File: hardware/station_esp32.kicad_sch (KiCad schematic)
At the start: 8 parts, among them J1 Conn_01x04, U1 DHT11, U2 ESP32-WROOM-32

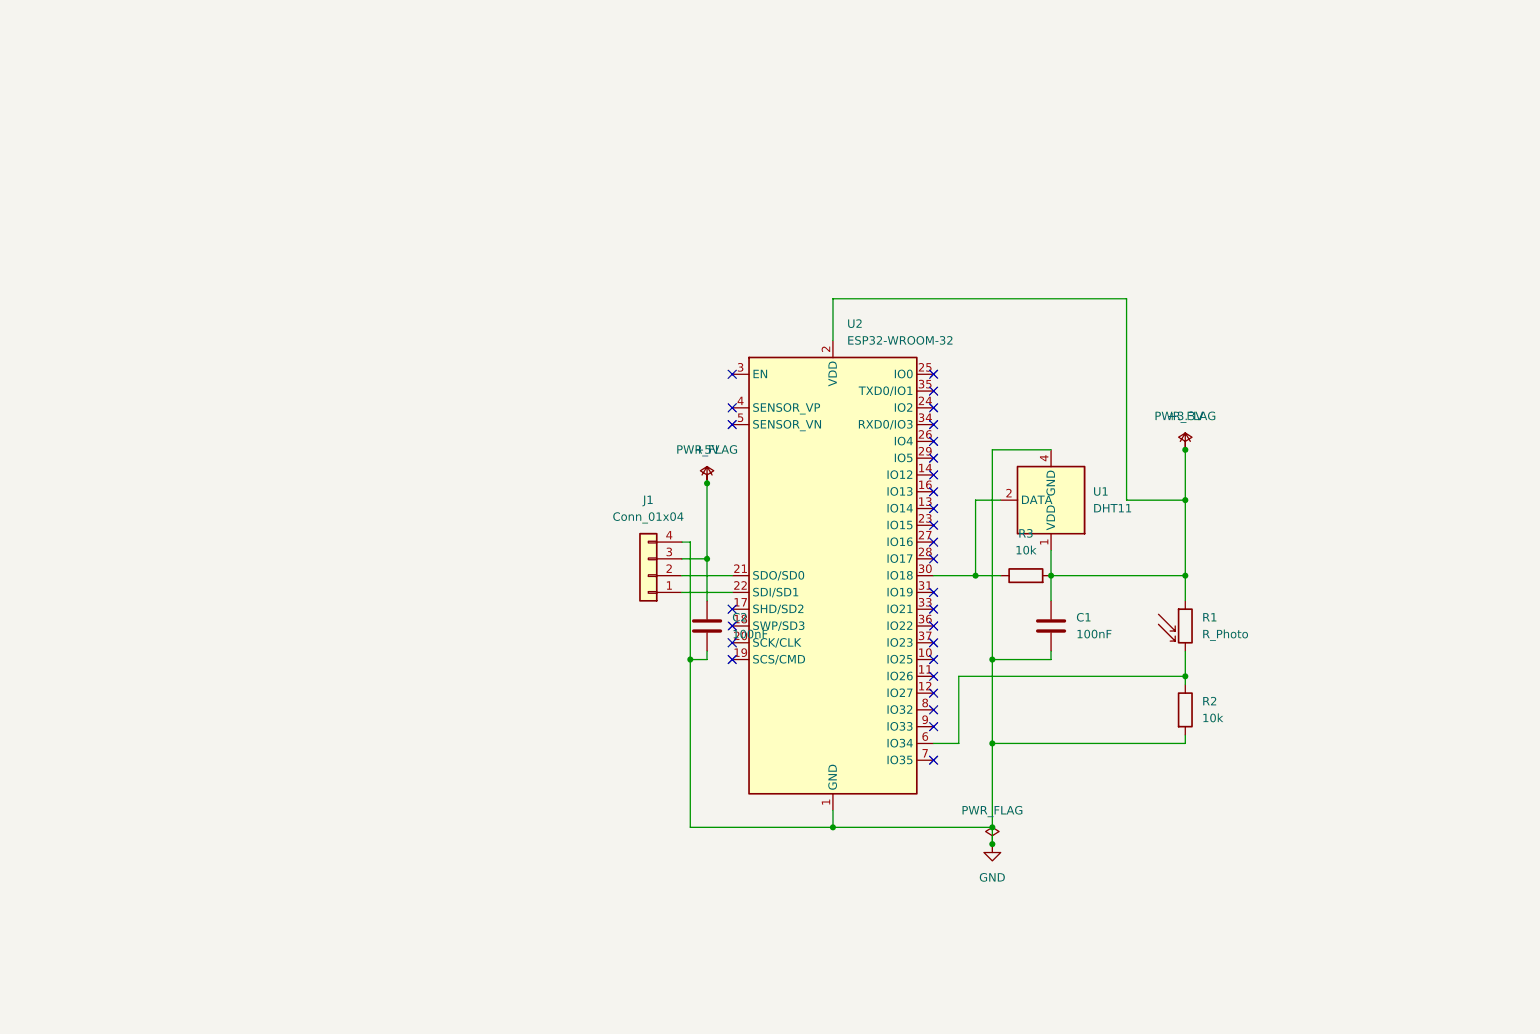
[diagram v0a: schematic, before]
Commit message: Add files via upload
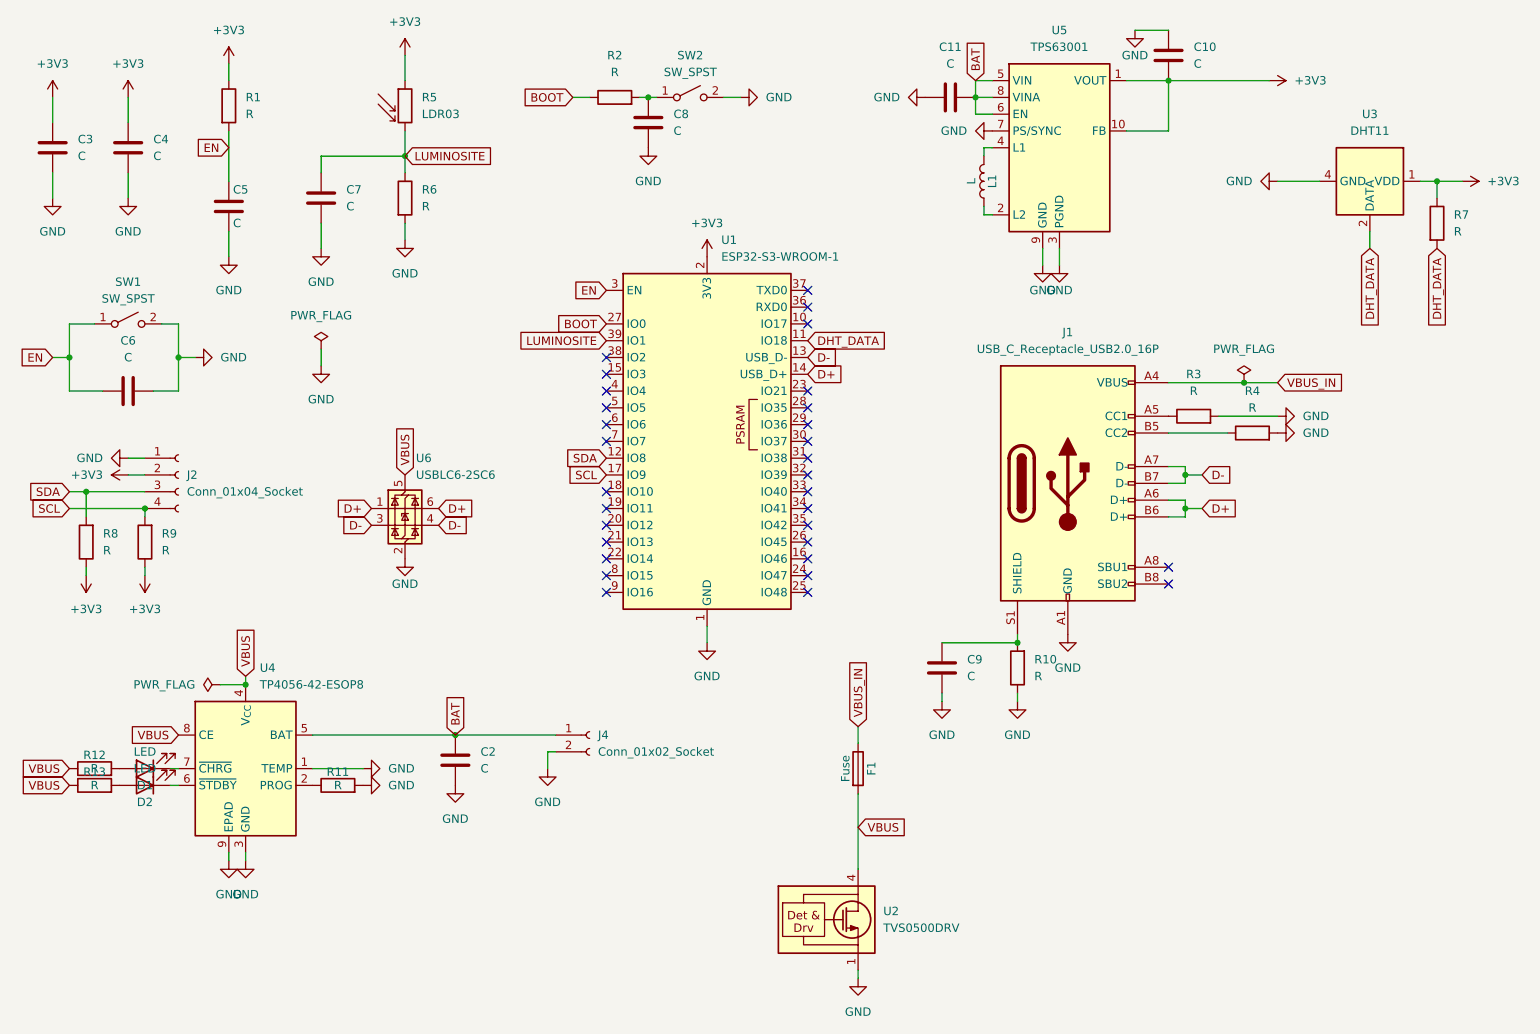
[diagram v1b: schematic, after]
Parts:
- removed C1: 100nF, Capacitor_THT:C_Disc_D5.0mm_W2.5mm_P5.00mm, symbol Device:C
- removed J1: Conn_01x04, Connector_PinHeader_2.54mm:PinHeader_1x04_P2.54mm_Vertical, symbol Connector_Generic:Conn_01x04
- removed R1: R_Photo, OptoDevice:R_LDR_5.0x4.1mm_P3mm_Vertical, symbol Device:R_Photo
- removed U1: DHT11, Sensor:Aosong_DHT11_5.5x12.0_P2.54mm, symbol Sensor:DHT11
- removed U2: ESP32-WROOM-32, RF_Module:ESP32-WROOM-32, symbol RF_Module:ESP32-WROOM-32
- added C10, C11, C3, C4, C5, C6, C7, C8, C9: C, Capacitor_SMD:C_0805_2012Metric, symbol Device:C
- added D1, D2: LED, LED_SMD:LED_0805_2012Metric, symbol Device:LED
- added F1: Fuse, Fuse:Fuse_0805_2012Metric, symbol Device:Fuse
- added J1: USB_C_Receptacle_USB2.0_16P, Connector_USB:USB_C_Receptacle_GCT_USB4105-xx-A_16P_TopMnt_Horizontal, symbol Connector:USB_C_Receptacle_USB2.0_16P
- added J2: Conn_01x04_Socket, Connector_JST:JST_PH_B4B-PH-K_1x04_P2.00mm_Vertical, symbol Connector:Conn_01x04_Socket
- added J4: Conn_01x02_Socket, Connector_JST:JST_PH_B2B-PH-K_1x02_P2.00mm_Vertical, symbol Connector:Conn_01x02_Socket
- added L1: L, Inductor_SMD:L_0805_2012Metric, symbol Device:L
- added R1, R10, R11, R12, R13, R4, R6, R7, R8, R9: R, Resistor_SMD:R_0805_2012Metric, symbol Device:R
- added R5: LDR03, OptoDevice:R_LDR_10x8.5mm_P7.6mm_Vertical, symbol Sensor_Optical:LDR03
- added SW1, SW2: SW_SPST, Button_Switch_SMD:SW_SPST_B3U-1000P, symbol Switch:SW_SPST
- added U1: ESP32-S3-WROOM-1, RF_Module:ESP32-S3-WROOM-1, symbol RF_Module:ESP32-S3-WROOM-1
- added U2: TVS0500DRV, Package_SON:WSON-6-1EP_2x2mm_P0.65mm_EP1x1.6mm, symbol Power_Protection:TVS0500DRV
- added U3: DHT11, Sensor:Aosong_DHT11_5.5x12.0_P2.54mm, symbol Sensor:DHT11
- added U4: TP4056-42-ESOP8, Package_SO:SOIC-8-1EP_3.9x4.9mm_P1.27mm_EP2.41x3.3mm_ThermalVias, symbol Battery_Management:TP4056-42-ESOP8
- added U5: TPS63001, Package_SON:Texas_DRC0010J_ThermalVias, symbol Regulator_Switching:TPS63001
- added U6: USBLC6-2SC6, Package_TO_SOT_SMD:SOT-23-6, symbol Power_Protection:USBLC6-2SC6
- C2: value 100nF -> C; footprint Capacitor_THT:C_Disc_D5.0mm_W2.5mm_P5.00mm -> Capacitor_SMD:C_0805_2012Metric
- R2, R3: value 10k -> R; footprint Resistor_THT:R_Axial_DIN0207_L6.3mm_D2.5mm_P10.16mm_Horizontal -> Resistor_SMD:R_0805_2012Metric
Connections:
- net +3.3V is gone; now on net GND: R3.2
- net GND: now also C10.1, C11.1, C3.2, C4.2, C5.2, C6.2, C7.2, C8.2, C9.2, J1.A1 (GND), J1.A12 (GND), J1.B1 (GND), J1.B12 (GND), J2.1 (Pin_1), J4.2 (Pin_2), R10.1, R11.2, R4.2, R6.2, SW1.2 (B), SW2.2 (B), U1.1 (GND), U1.40 (GND), U1.41 (GND), U2.1 (GND), U2.2 (GND), U2.3 (GND), U2.7 (GND), U3.4 (GND), U4.1 (TEMP), U4.3 (GND), U4.9 (EPAD), U5.11 (PGND), U5.3 (PGND), U5.7 (PS/SYNC), U5.9 (GND), U6.2 (GND); no longer R2.2
- net BOOT: now reaches R2.1
- net BOOT: now also U1.27 (IO0)
- net at R3.1: now also J1.A5 (CC1)
- net +5V renamed BAT
- net BAT: now also C11.2, J4.1 (Pin_1), U4.5 (BAT), U5.5 (VIN), U5.6 (EN), U5.8 (VINA)
- new net: C8.1, R2.2, SW2.1 (A)
- new net: D2.2 (A), R13.2
- new net: L1.1, U5.2 (L2)
- new net: L1.2, U5.4 (L1)
- new net: R11.1, U4.2 (PROG)
- new net: D1.2 (A), R12.2
- new net: D1.1 (K), U4.7 (~{CHRG})
- new net: J1.B5 (CC2), R4.1
- new net: C9.1, J1.S1 (SHIELD), R10.2
- new net: D2.1 (K), U4.6 (~{STDBY})
- new net +3V3: C10.2, C3.1, C4.1, J2.2 (Pin_2), R1.1, R5.1, R7.1, R8.1, R9.1, U1.2 (3V3), U3.1 (VDD), U5.1 (VOUT), U5.10 (FB)
- new net D+: J1.A6 (D+), J1.B6 (D+), U1.14 (USB_D+), U6.1 (I/O1), U6.6 (I/O1)
- new net D-: J1.A7 (D-), J1.B7 (D-), U1.13 (USB_D-), U6.3 (I/O2), U6.4 (I/O2)
- new net DHT_DATA: R7.2, U1.11 (IO18), U3.2 (DATA)
- new net EN: C5.1, C6.1, R1.2, SW1.1 (A), U1.3 (EN)
- new net LUMINOSITE: C7.1, R5.2, R6.1, U1.39 (IO1)
- new net SCL: J2.4 (Pin_4), R9.2, U1.17 (IO9)
- new net SDA: J2.3 (Pin_3), R8.2, U1.12 (IO8)
- new net VBUS: F1.2, R12.1, R13.1, U2.4 (IN), U2.5 (IN), U2.6 (IN), U4.4 (V_{CC}), U4.8 (CE), U6.5 (VBUS)
- new net VBUS_IN: F1.1, J1.A4 (VBUS), J1.A9 (VBUS), J1.B4 (VBUS), J1.B9 (VBUS)
- no-connect marks 29 -> 31
